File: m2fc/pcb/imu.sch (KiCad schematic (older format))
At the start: 49 parts

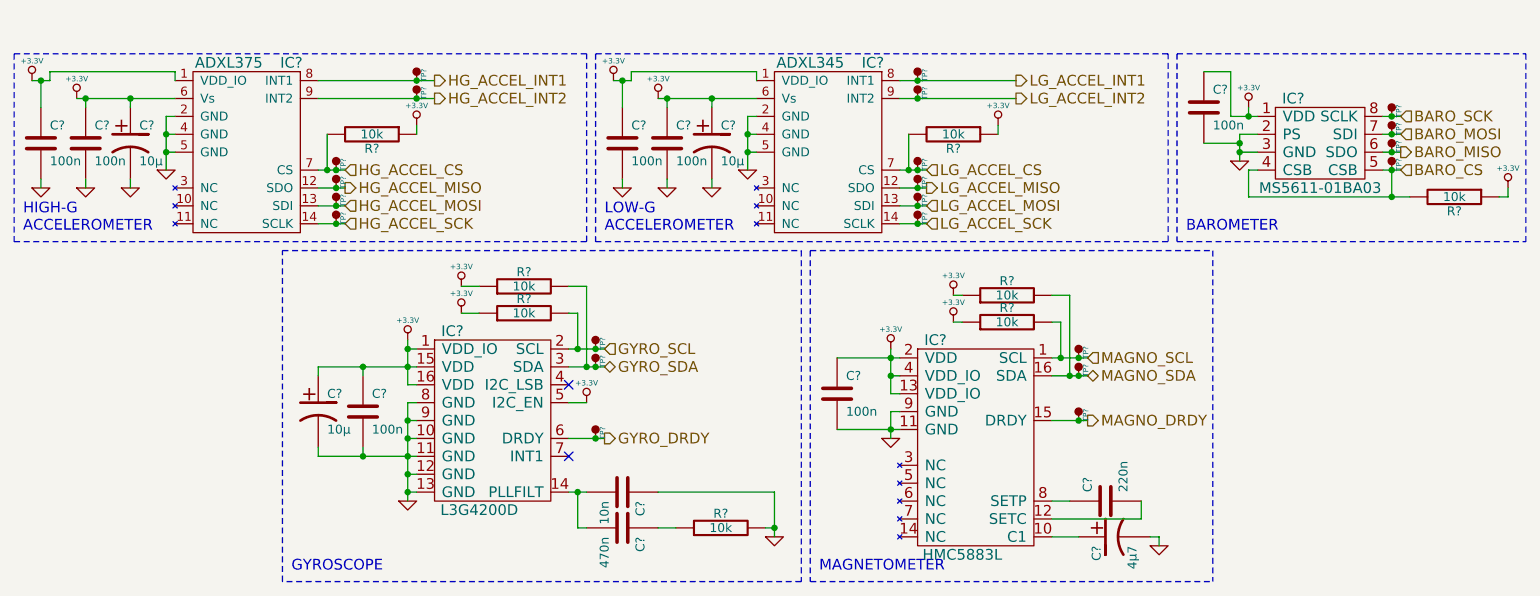
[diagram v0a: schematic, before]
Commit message: update more bits on flight computer..
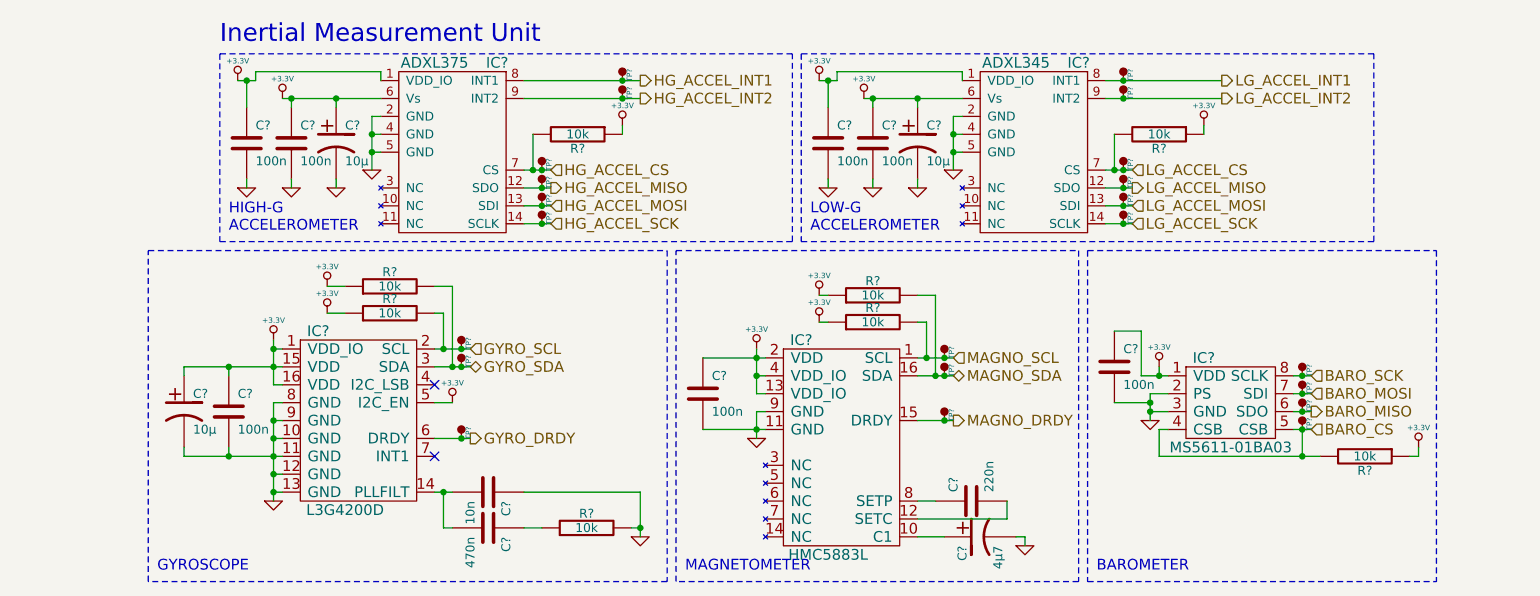
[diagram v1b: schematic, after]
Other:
- note added: "Inertial Measurement Unit"
- moved on the sheet: C?, IC?, R?, TP?
